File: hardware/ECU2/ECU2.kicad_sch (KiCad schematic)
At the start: 31 parts, among them J1 Conn_fuel, J2 Conn_speed, J3 Conn_fuel_gauge, J4 Conn_RPM, U1 step down (buck), U2 ESP32-WROOM-32

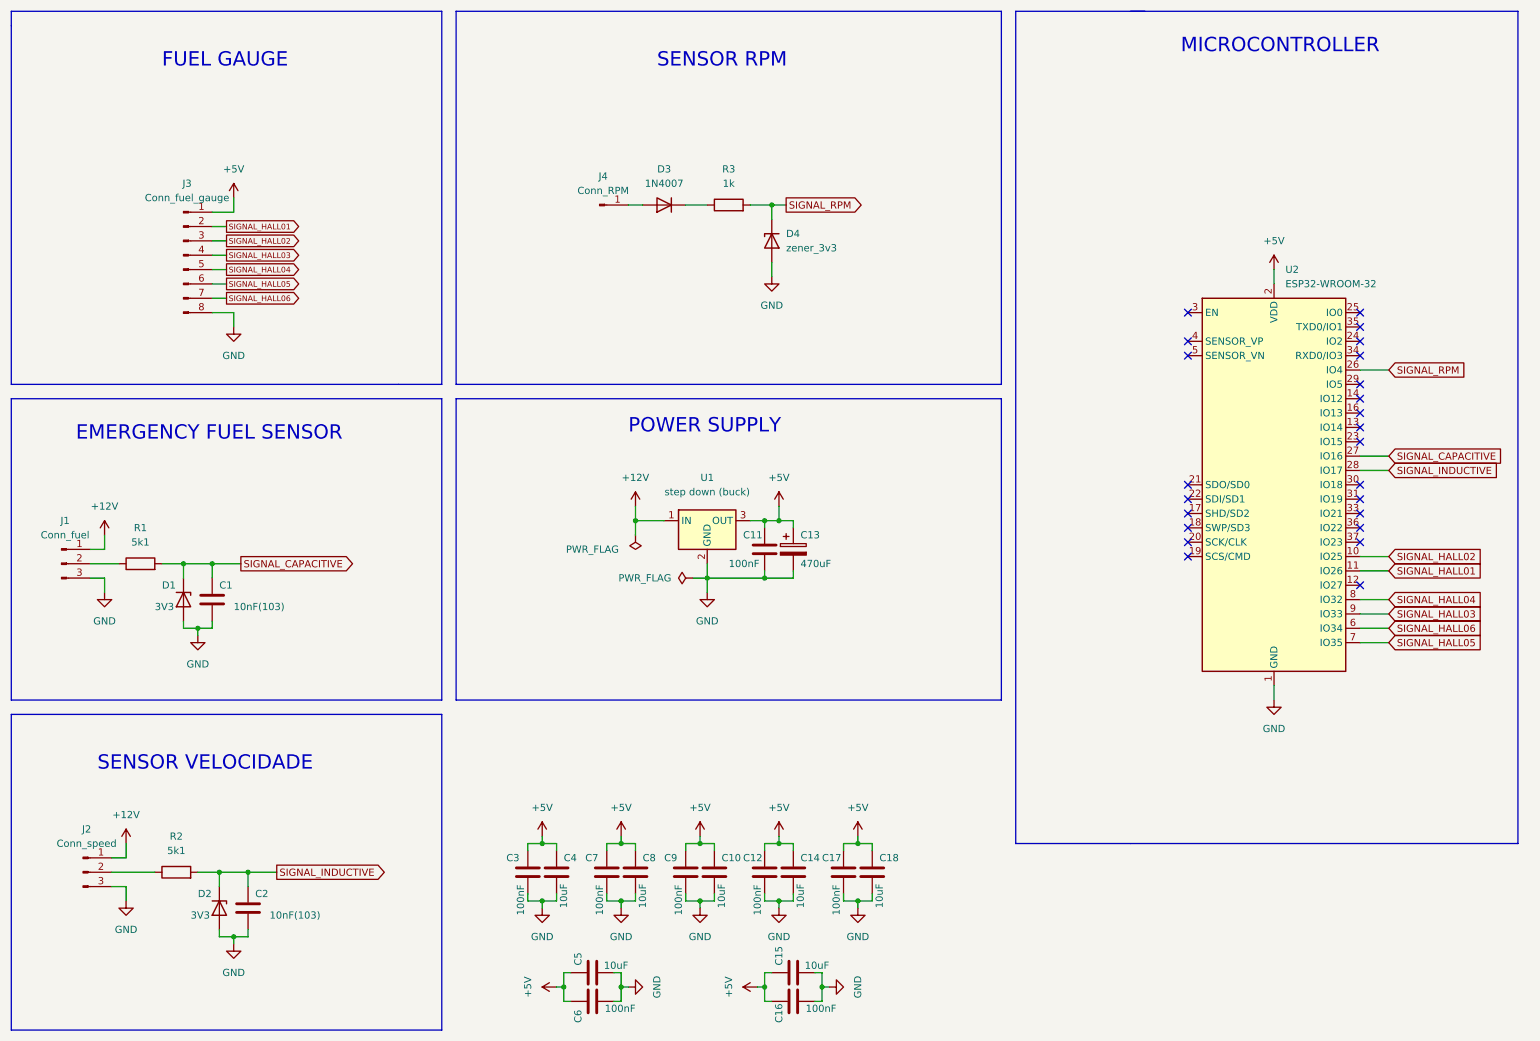
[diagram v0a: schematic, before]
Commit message: add images to README
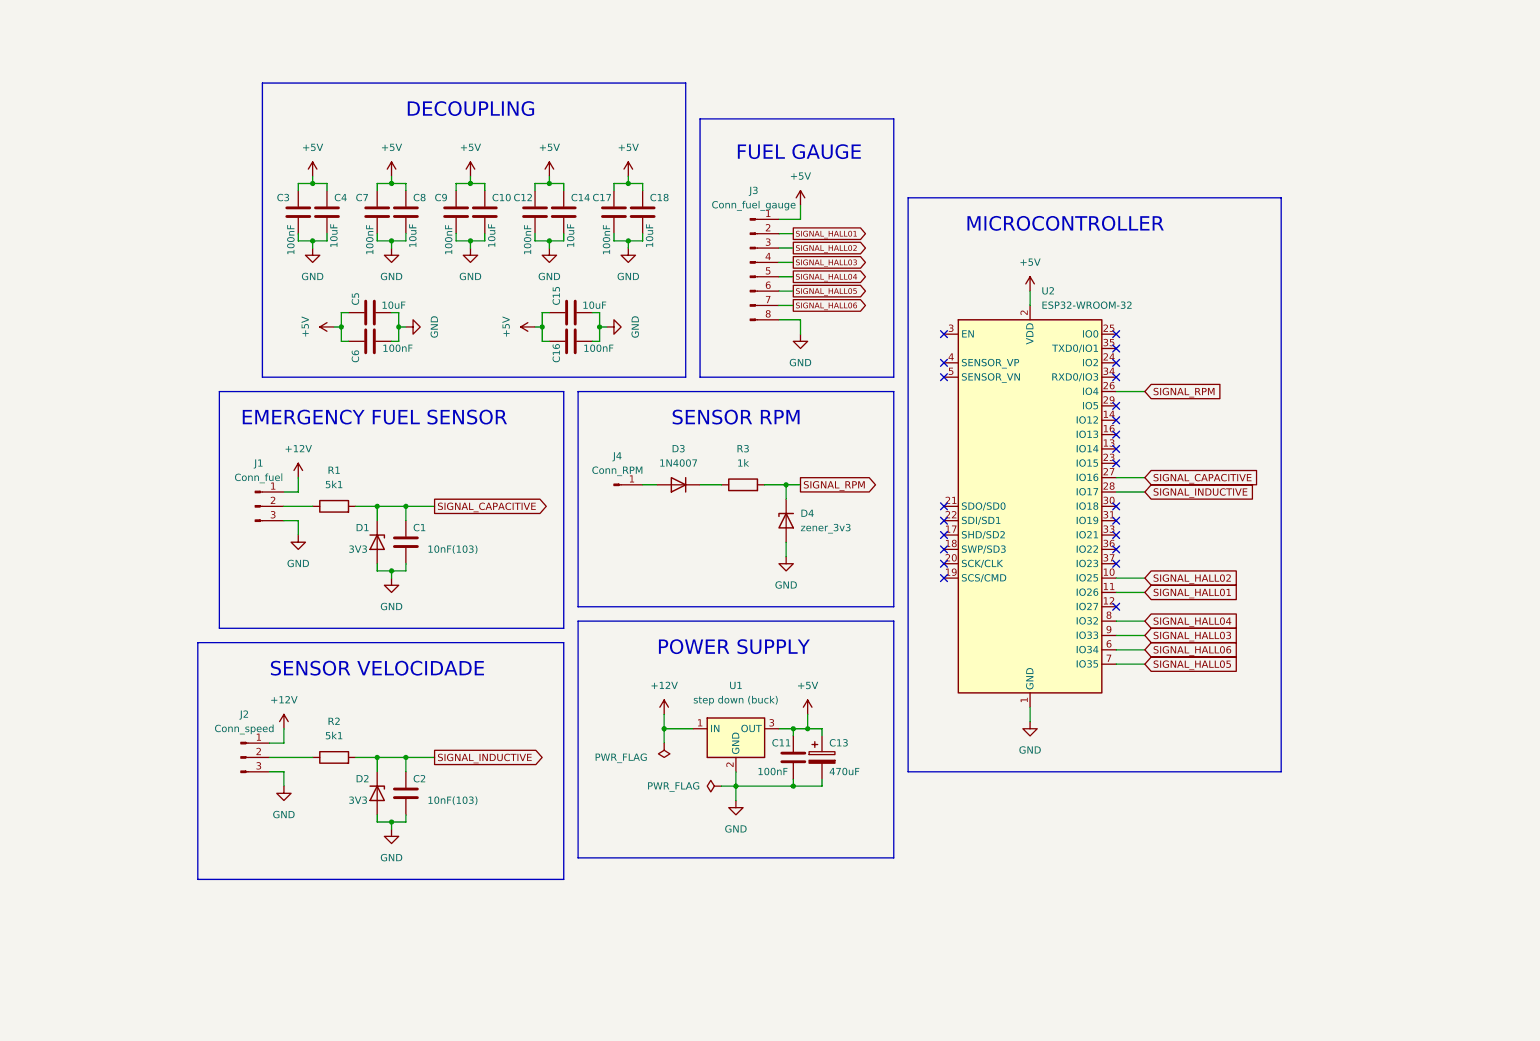
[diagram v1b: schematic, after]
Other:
- note added: "DECOUPLING"
- moved on the sheet: C1, C10, C11, C12, C13, C14, C15, C16, C17, C18, C2, C3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
